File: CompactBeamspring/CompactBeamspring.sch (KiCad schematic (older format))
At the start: 32 parts, among them J1 BEAMSPRING CONNECTOR, J2 PadsToShort, J3 EXPANSION HEADER, U1 MCP4921-E, U2 LM339A, U3 74AHC595, U4 74AHC595, U5 ProMicro, U7 74AHC595

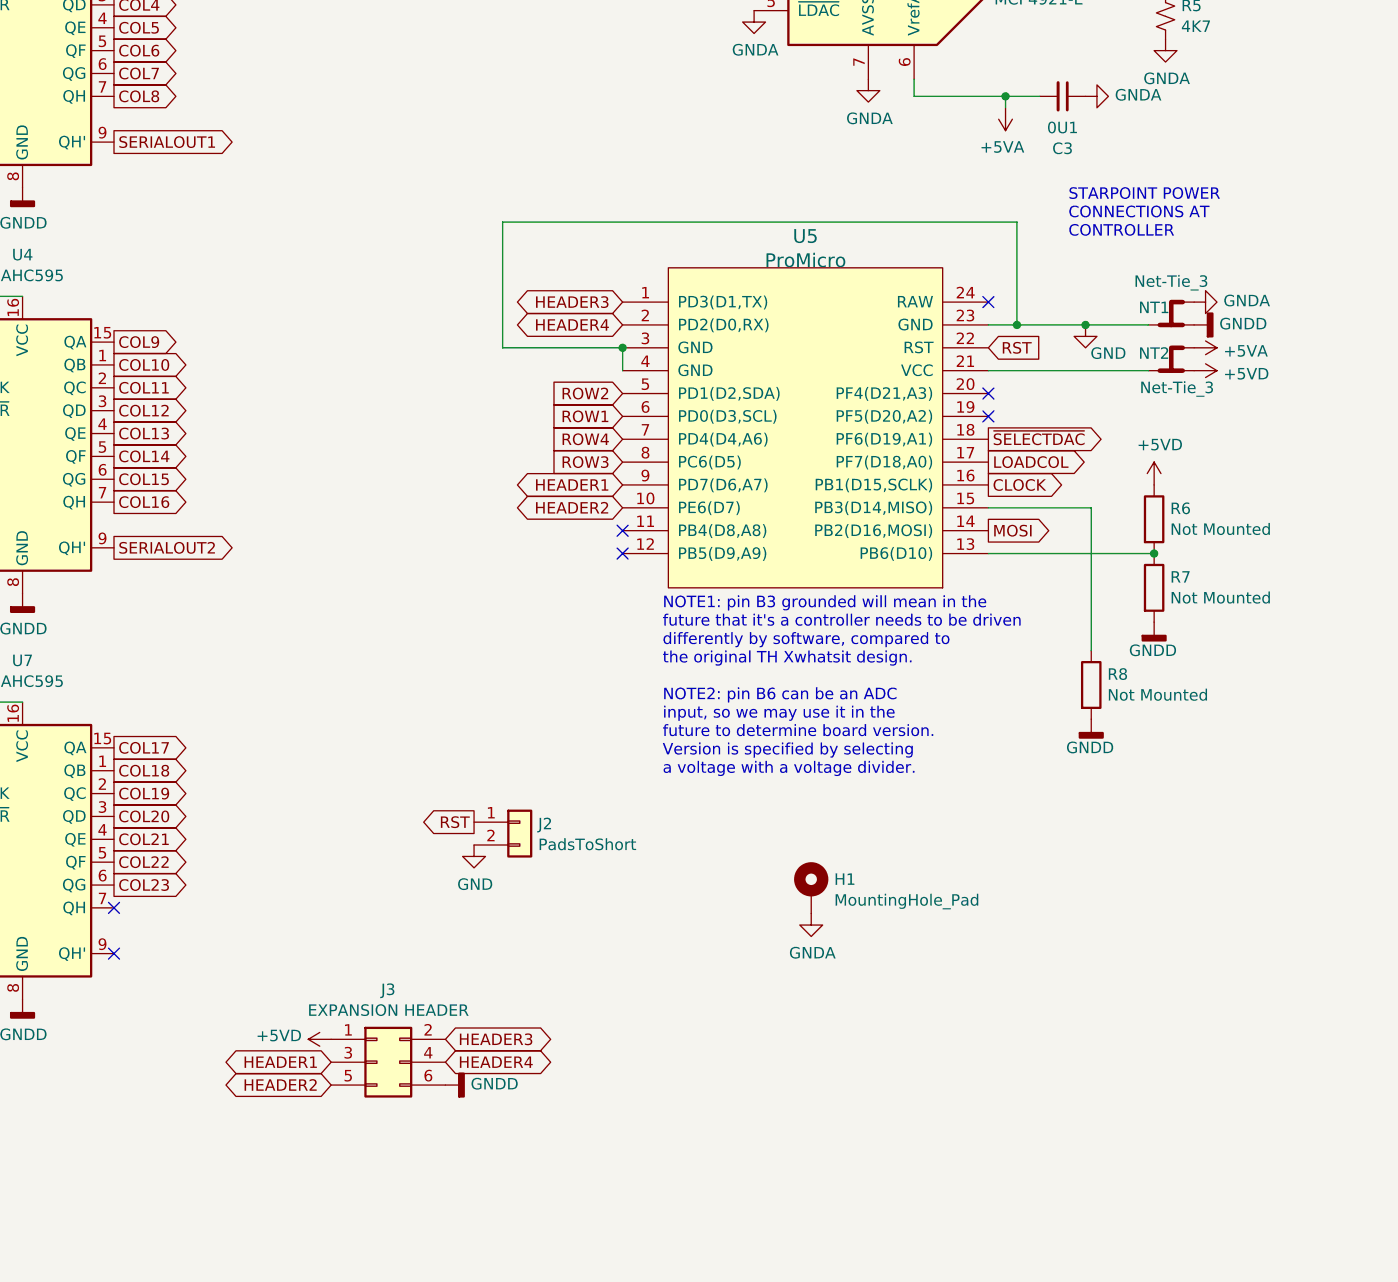
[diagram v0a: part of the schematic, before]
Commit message: Updated to rev. 1.4
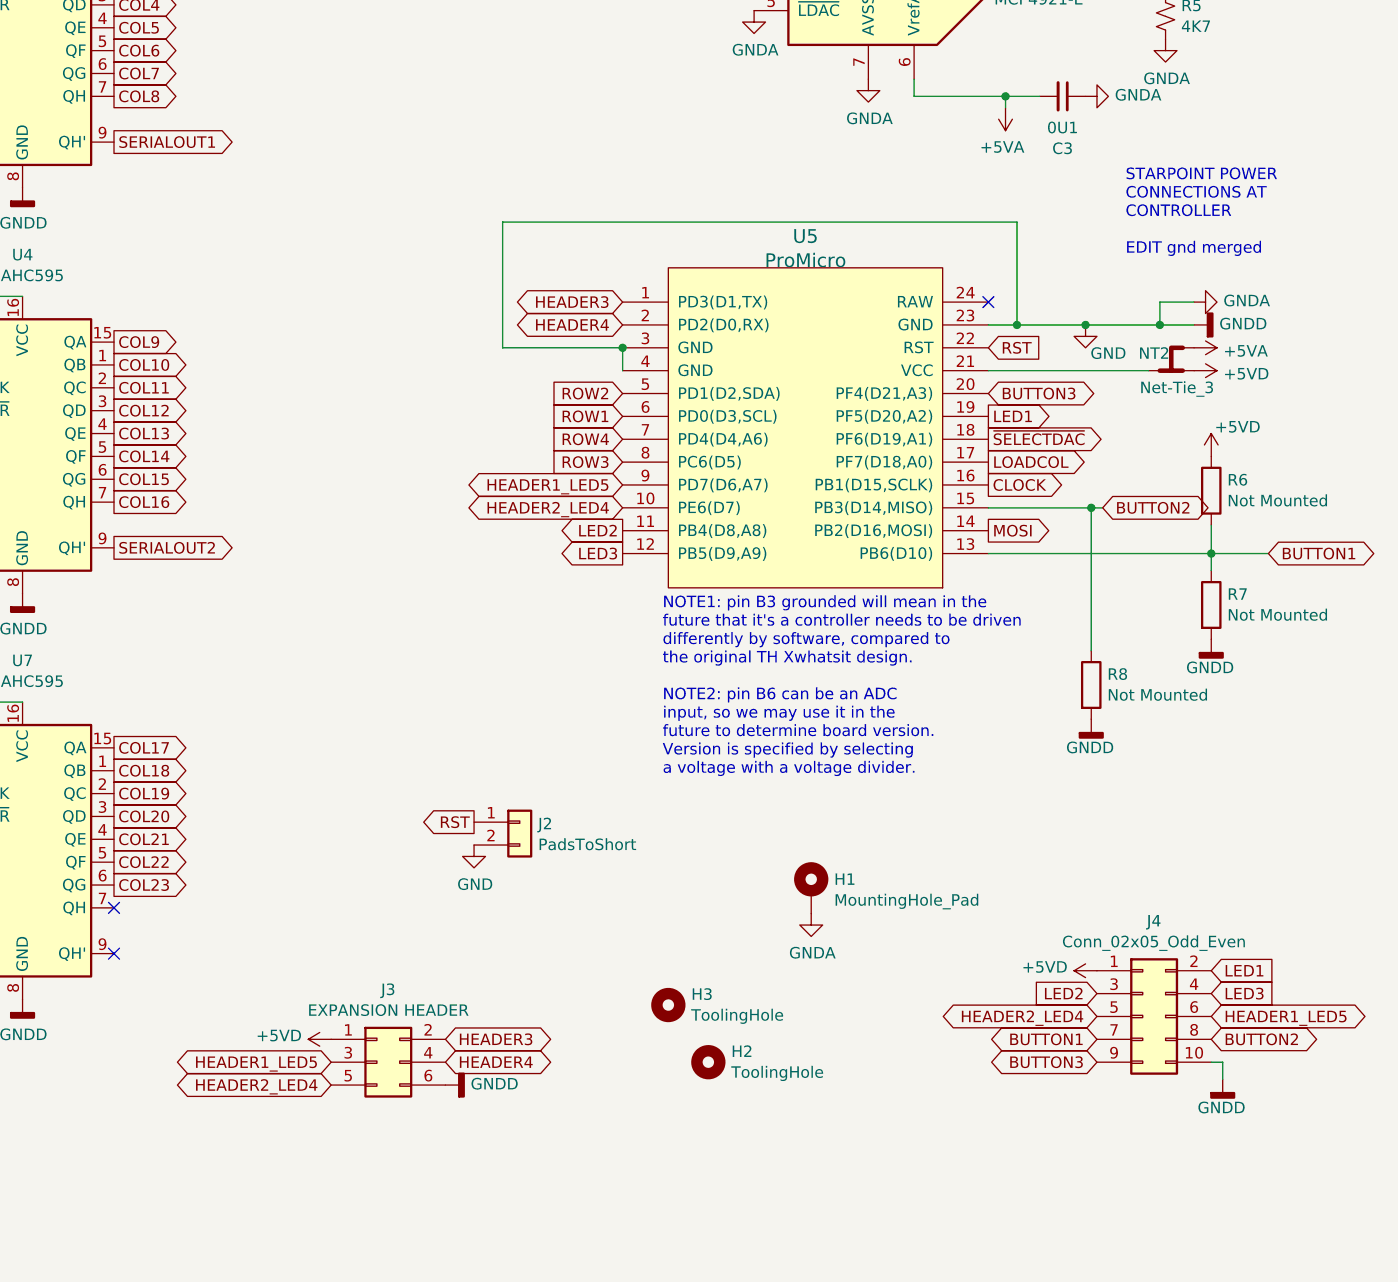
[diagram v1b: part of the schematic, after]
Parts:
- removed NT1: Net-Tie_3, NetTie:NetTie-3_THT_Pad0.3mm, symbol Device:Net-Tie_3
- added H2, H3: ToolingHole, TH-XWhatsIt:tooling_hole, symbol Mechanical:MountingHole
- added J4: Conn_02x05_Odd_Even, Connector_PinHeader_2.54mm:PinHeader_2x05_P2.54mm_Vertical, symbol Connector_Generic:Conn_02x05_Odd_Even
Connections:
- net GNDA is gone; now on net GND: C1.1, C3.1, C6.1, H1.1, R2.1, R5.1, U1.5 (~LDAC~), U1.7 (AVSS), U2.12 (V-)
- net GNDD is gone; now on net GND: C2.1, C4.1, C5.1, J1.30 (Pin_30), J1.5 (Pin_5), J3.6 (Pin_6), R7.2, R8.2, U3.13 (~OE), U3.8 (GND), U4.13 (~OE), U4.8 (GND), U7.13 (~OE), U7.8 (GND)
- net +5VD: now also J4.1 (Pin_1)
- net GND: now also J4.10 (Pin_10)
- net LED2: now reaches U5.11 (PB4(D8,A8))
- net LED2: now also J4.3 (Pin_3)
- net LED3: now reaches U5.12 (PB5(D9,A9))
- net LED3: now also J4.4 (Pin_4)
- net BUTTON1: now reaches R6.2, R7.1, U5.13 (PB6(D10))
- net BUTTON1: now also J4.7 (Pin_7)
- net BUTTON2: now reaches R8.1, U5.15 (PB3(D14,MISO))
- net BUTTON2: now also J4.8 (Pin_8)
- net LED1: now reaches U5.19 (PF5(D20,A2))
- net LED1: now also J4.2 (Pin_2)
- net BUTTON3: now reaches U5.20 (PF4(D21,A3))
- net BUTTON3: now also J4.9 (Pin_9)
- net HEADER1 renamed HEADER1_LED5
- net HEADER1_LED5: now also J4.6 (Pin_6)
- net HEADER2 renamed HEADER2_LED4
- net HEADER2_LED4: now also J4.5 (Pin_5)
- no-connect marks 8 -> 4
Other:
- note added: "STARPOINT POWER\nCONNECTIONS AT\nCONTROLLER\n\nEDIT gnd merged"
- note removed: "STARPOINT POWER\nCONNECTIONS AT\nCONTROLLER"
- moved on the sheet: R7
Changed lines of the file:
@@
 Title "Compact Beamspring Controller Based on TH Xwhatsit"
 Date "2020-01-31"
-Rev "1.3"
+Rev "1.4"
 Comp "Rainy Day Plans"
 Comment1 ""
@@
 HEADER4
 Text GLabel 7900 3575 0    50   BiDi ~ 0
-HEADER1
+HEADER1_LED5
 Text GLabel 7900 3675 0    50   BiDi ~ 0
-HEADER2
+HEADER2_LED4
 Text GLabel 7900 2775 0    50   BiDi ~ 0
 HEADER3
@@
 HEADER4
 Text GLabel 6625 6200 0    50   BiDi ~ 0
-HEADER2
+HEADER2_LED4
 Text GLabel 6625 6100 0    50   BiDi ~ 0
-HEADER1
+HEADER1_LED5
 Text Notes 3950 7750 0    50   ~ 0
 Copyright Rainy Day Plans.\nThis documentation describes Open Hardware and is licensed under the\nCERN OHL v. 1.2.\nYou may redistribute and modify this documentation under the terms of the\nCERN OHL v.1.2. (http://ohwr.org/cernohl). This documentation is distributed\nWITHOUT ANY EXPRESS OR IMPLIED WARRANTY, INCLUDING OF\nMERCHANTABILITY, SATISFACTORY QUALITY AND FITNESS FOR A\nPARTICULAR PURPOSE. Please see the CERN OHL v.1.2 for applicable\nconditions
@@
 L power:GNDD #PWR0107
 U 1 1 5F3A2D72
-P 10225 4175
-F 0 "#PWR0107" H 10225 3925 50  0001 C CNN
-F 1 "GNDD" H 10325 4050 50  0000 R CNN
-F 2 "" H 10225 4175 50  0001 C CNN
-F 3 "" H 10225 4175 50  0001 C CNN
-	1    10225 4175
+P 10475 4250
+F 0 "#PWR0107" H 10475 4000 50  0001 C CNN
+F 1 "GNDD" H 10575 4125 50  0000 R CNN
+F 2 "" H 10475 4250 50  0001 C CNN
+F 3 "" H 10475 4250 50  0001 C CNN
+	1    10475 4250
 	1    0    0    -1
 $EndComp
@@
 	2250 4275 2250 4300
 $Comp
-L Device:Net-Tie_3 NT1
-U 1 1 5F6D07D8
-P 10300 2875
-F 0 "NT1" H 10375 2800 50  0000 C CNN
-F 1 "Net-Tie_3" H 10300 2685 50  0000 C CNN
-F 2 "NetTie:NetTie-3_THT_Pad0.3mm" H 10300 2875 50  0001 C CNN
-F 3 "~" H 10300 2875 50  0001 C CNN
-	1    10300 2875
-	-1   0    0    1
-$EndComp
-$Comp
 L Device:Net-Tie_3 NT2
 U 1 1 5F6D1B28
@@
 	9625 2875 9500 2875
 $Comp
-L Device:R R6
-U 1 1 5F3A43C9
-P 10225 3725
-F 0 "R6" H 10295 3771 50  0000 L CNN
-F 1 "Not Mounted" H 10295 3680 50  0000 L CNN
-F 2 "Resistor_SMD:R_0805_2012Metric_Pad1.15x1.40mm_HandSolder" V 10155 3725 50  0001 C CNN
-F 3 "~" H 10225 3725 50  0001 C CNN
-	1    10225 3725
-	1    0    0    -1
-$EndComp
-$Comp
 L Device:R R7
 U 1 1 5F3A4C74
-P 10225 4025
-F 0 "R7" H 10295 4071 50  0000 L CNN
-F 1 "Not Mounted" H 10295 3980 50  0000 L CNN
-F 2 "Resistor_SMD:R_0805_2012Metric_Pad1.15x1.40mm_HandSolder" V 10155 4025 50  0001 C CNN
-F 3 "~" H 10225 4025 50  0001 C CNN
-	1    10225 4025
-	1    0    0    -1
-$EndComp
-Connection ~ 10225 3875
-$Comp
-L power:+5VD #PWR04
-U 1 1 5F3A9745
-P 10225 3575
-F 0 "#PWR04" H 10225 3425 50  0001 C CNN
-F 1 "+5VD" H 10150 3750 50  0000 L CNN
-F 2 "" H 10225 3575 50  0001 C CNN
-F 3 "" H 10225 3575 50  0001 C CNN
-	1    10225 3575
+P 10475 4100
+F 0 "R7" H 10545 4146 50  0000 L CNN
+F 1 "Not Mounted" H 10545 4055 50  0000 L CNN
+F 2 "Resistor_SMD:R_0805_2012Metric_Pad1.15x1.40mm_HandSolder" V 10405 4100 50  0001 C CNN
+F 3 "~" H 10475 4100 50  0001 C CNN
+	1    10475 4100
 	1    0    0    -1
 $EndComp
@@
 Wire Wire Line
 	9950 4300 9950 3675
-NoConn ~ 9500 3175
-NoConn ~ 9500 3275
-NoConn ~ 7900 3775
-NoConn ~ 7900 3875
 $Comp
 L Connector_Generic:Conn_01x02 J2
@@
 Text GLabel 7250 5050 0    50   Output ~ 0
 RST
-Wire Wire Line
-	10200 2875 9925 2875
 Connection ~ 9925 2875
 $Comp
@@
 	1    0    0    -1
 $EndComp
-Text Notes 9850 2500 0    50   ~ 0
-STARPOINT POWER\nCONNECTIONS AT\nCONTROLLER
+Text Notes 10100 2575 0    50   ~ 0
+STARPOINT POWER\nCONNECTIONS AT\nCONTROLLER\n\nEDIT gnd merged
 $Comp
 L power:GND #PWR08
@@
 	9500 3075 10200 3075
 Wire Wire Line
-	9500 3875 10225 3875
-Wire Wire Line
 	9500 3675 9950 3675
 Wire Wire Line
@@
 Wire Wire Line
 	7375 2425 9625 2425
+$Comp
+L Connector_Generic:Conn_02x05_Odd_Even J4
+U 1 1 6107AC92
+P 10175 5900
+F 0 "J4" H 10225 6317 50  0000 C CNN
+F 1 "Conn_02x05_Odd_Even" H 10225 6226 50  0000 C CNN
+F 2 "Connector_PinHeader_2.54mm:PinHeader_2x05_P2.54mm_Vertical" H 10175 5900 50  0001 C CNN
+F 3 "~" H 10175 5900 50  0001 C CNN
+	1    10175 5900
+	1    0    0    -1
+$EndComp
+Wire Wire Line
+	9925 2875 10250 2875
+Wire Wire Line
+	10250 2875 10250 2775
+Wire Wire Line
+	10250 2775 10400 2775
+Connection ~ 10250 2875
+Wire Wire Line
+	10250 2875 10400 2875
+$Comp
+L power:+5VD #PWR04
+U 1 1 61088086
+P 9975 5700
+F 0 "#PWR04" H 9975 5550 50  0001 C CNN
+F 1 "+5VD" V 9990 5828 50  0000 L CNN
+F 2 "" H 9975 5700 50  0001 C CNN
+F 3 "" H 9975 5700 50  0001 C CNN
+	1    9975 5700
+	0    -1   -1   0
+$EndComp
+Text GLabel 9500 3275 2    50   Output ~ 0
+LED1
+Text GLabel 10475 5700 2    50   Input ~ 0
+LED1
+Text GLabel 7900 3775 0    50   Output ~ 0
+LED2
+Text GLabel 7900 3875 0    50   Output ~ 0
+LED3
+Text GLabel 9975 5800 0    50   Input ~ 0
+LED2
+Text GLabel 10475 5800 2    50   Input ~ 0
+LED3
+Text GLabel 9975 5900 0    50   BiDi ~ 0
+HEADER2_LED4
+Text GLabel 10475 5900 2    50   BiDi ~ 0
+HEADER1_LED5
+Text GLabel 10725 3875 2    50   BiDi ~ 0
+BUTTON1
+Text GLabel 9975 6000 0    50   BiDi ~ 0
+BUTTON1
+Text GLabel 10000 3675 2    50   BiDi ~ 0
+BUTTON2
+Text GLabel 10475 6000 2    50   BiDi ~ 0
+BUTTON2
+Text GLabel 9500 3175 2    50   BiDi ~ 0
+BUTTON3
+Text GLabel 9975 6100 0    50   BiDi ~ 0
+BUTTON3
+$Comp
+L Device:R R6
+U 1 1 610C2CCF
+P 10475 3600
+F 0 "R6" H 10545 3646 50  0000 L CNN
+F 1 "Not Mounted" H 10545 3555 50  0000 L CNN
+F 2 "Resistor_SMD:R_0805_2012Metric_Pad1.15x1.40mm_HandSolder" V 10405 3600 50  0001 C CNN
+F 3 "~" H 10475 3600 50  0001 C CNN
+	1    10475 3600
+	1    0    0    -1
+$EndComp
+$Comp
+L power:GNDD #PWR0103
+U 1 1 610D5B38
+P 10525 6175
+F 0 "#PWR0103" H 10525 5925 50  0001 C CNN
+F 1 "GNDD" H 10625 6050 50  0000 R CNN
+F 2 "" H 10525 6175 50  0001 C CNN
+F 3 "" H 10525 6175 50  0001 C CNN
+	1    10525 6175
+	1    0    0    -1
+$EndComp
+Wire Wire Line
+	10475 6100 10525 6100
+Wire Wire Line
+	10525 6100 10525 6175
+Wire Wire Line
+	10000 3675 9950 3675
+Connection ~ 9950 3675
+Wire Wire Line
+	9500 3875 10475 3875
+Wire Wire Line
+	10475 3750 10475 3875
+Connection ~ 10475 3875
+Wire Wire Line
+	10475 3875 10725 3875
+Wire Wire Line
+	10475 3875 10475 3950
+$Comp
+L power:+5VD #PWR0110
+U 1 1 6112E48C
+P 10475 3450
+F 0 "#PWR0110" H 10475 3300 50  0001 C CNN
+F 1 "+5VD" H 10490 3578 50  0000 L CNN
+F 2 "" H 10475 3450 50  0001 C CNN
+F 3 "" H 10475 3450 50  0001 C CNN
+	1    10475 3450
+	1    0    0    -1
+$EndComp
+$Comp
+L Mechanical:MountingHole H2
+U 1 1 611D25F7
+P 8275 6100
+F 0 "H2" H 8375 6146 50  0000 L CNN
+F 1 "ToolingHole" H 8375 6055 50  0000 L CNN
+F 2 "TH-XWhatsIt:tooling_hole" H 8275 6100 50  0001 C CNN
+F 3 "~" H 8275 6100 50  0001 C CNN
+	1    8275 6100
+	1    0    0    -1
+$EndComp
+$Comp
+L Mechanical:MountingHole H3
+U 1 1 611DB711
+P 8100 5850
+F 0 "H3" H 8200 5896 50  0000 L CNN
+F 1 "ToolingHole" H 8200 5805 50  0000 L CNN
+F 2 "TH-XWhatsIt:tooling_hole" H 8100 5850 50  0001 C CNN
+F 3 "~" H 8100 5850 50  0001 C CNN
+	1    8100 5850
+	1    0    0    -1
+$EndComp
 $EndSCHEMATC

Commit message: Updated shift register and 100k resistor LCSC part numbers
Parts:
- R10, R11, R12, R9: LCSC C17407 -> C149504
- U3, U4, U7: LCSC C5520 -> C2682116
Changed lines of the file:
@@
 F 2 "Package_SO:SOIC-16_3.9x9.9mm_P1.27mm" H 5275 1575 50  0001 C CNN
 F 3 "https://assets.nexperia.com/documents/data-sheet/74HC_HCT595.pdf" H 5275 1575 50  0001 C CNN
-F 4 "C5520" H 5275 1575 50  0001 C CNN "LCSC"
+F 4 "C2682116" H 5275 1575 50  0001 C CNN "LCSC"
 	1    5275 1575
 	1    0    0    -1
@@
 F 2 "Package_SO:SOIC-16_3.9x9.9mm_P1.27mm" H 5275 3350 50  0001 C CNN
 F 3 "https://assets.nexperia.com/documents/data-sheet/74HC_HCT595.pdf" H 5275 3350 50  0001 C CNN
-F 4 "C5520" H 5275 3350 50  0001 C CNN "LCSC"
+F 4 "C2682116" H 5275 3350 50  0001 C CNN "LCSC"
 	1    5275 3350
 	1    0    0    -1
@@
 F 2 "Package_SO:SOIC-16_3.9x9.9mm_P1.27mm" H 5275 5125 50  0001 C CNN
 F 3 "https://assets.nexperia.com/documents/data-sheet/74HC_HCT595.pdf" H 5275 5125 50  0001 C CNN
-F 4 "C5520" H 5275 5125 50  0001 C CNN "LCSC"
+F 4 "C2682116" H 5275 5125 50  0001 C CNN "LCSC"
 	1    5275 5125
 	1    0    0    -1
@@
 F 2 "Resistor_SMD:R_0805_2012Metric_Pad1.15x1.40mm_HandSolder" V 1380 1325 50  0001 C CNN
 F 3 "~" H 1450 1325 50  0001 C CNN
-F 4 "C17407" H 1450 1325 50  0001 C CNN "LCSC"
+F 4 "C149504" H 1450 1325 50  0001 C CNN "LCSC"
 	1    1450 1325
 	1    0    0    -1
@@
 F 2 "Resistor_SMD:R_0805_2012Metric_Pad1.15x1.40mm_HandSolder" V 1380 1925 50  0001 C CNN
 F 3 "~" H 1450 1925 50  0001 C CNN
-F 4 "C17407" H 1450 1925 50  0001 C CNN "LCSC"
+F 4 "C149504" H 1450 1925 50  0001 C CNN "LCSC"
 	1    1450 1925
 	1    0    0    -1
@@
 F 2 "Resistor_SMD:R_0805_2012Metric_Pad1.15x1.40mm_HandSolder" V 1380 2525 50  0001 C CNN
 F 3 "~" H 1450 2525 50  0001 C CNN
-F 4 "C17407" H 1450 2525 50  0001 C CNN "LCSC"
+F 4 "C149504" H 1450 2525 50  0001 C CNN "LCSC"
 	1    1450 2525
 	1    0    0    -1
@@
 F 2 "Resistor_SMD:R_0805_2012Metric_Pad1.15x1.40mm_HandSolder" V 1380 3125 50  0001 C CNN
 F 3 "~" H 1450 3125 50  0001 C CNN
-F 4 "C17407" H 1450 3125 50  0001 C CNN "LCSC"
+F 4 "C149504" H 1450 3125 50  0001 C CNN "LCSC"
 	1    1450 3125
 	1    0    0    -1

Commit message: Revert part of commit 'Updated 100k resistor and shift register LCSC part numbers' (the shift register BOM changes only)
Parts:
- U3, U4, U7: LCSC C2682116 -> C5520
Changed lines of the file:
@@
 F 2 "Package_SO:SOIC-16_3.9x9.9mm_P1.27mm" H 5275 1575 50  0001 C CNN
 F 3 "https://assets.nexperia.com/documents/data-sheet/74HC_HCT595.pdf" H 5275 1575 50  0001 C CNN
-F 4 "C2682116" H 5275 1575 50  0001 C CNN "LCSC"
+F 4 "C5520" H 5275 1575 50  0001 C CNN "LCSC"
 	1    5275 1575
 	1    0    0    -1
@@
 F 2 "Package_SO:SOIC-16_3.9x9.9mm_P1.27mm" H 5275 3350 50  0001 C CNN
 F 3 "https://assets.nexperia.com/documents/data-sheet/74HC_HCT595.pdf" H 5275 3350 50  0001 C CNN
-F 4 "C2682116" H 5275 3350 50  0001 C CNN "LCSC"
+F 4 "C5520" H 5275 3350 50  0001 C CNN "LCSC"
 	1    5275 3350
 	1    0    0    -1
@@
 F 2 "Package_SO:SOIC-16_3.9x9.9mm_P1.27mm" H 5275 5125 50  0001 C CNN
 F 3 "https://assets.nexperia.com/documents/data-sheet/74HC_HCT595.pdf" H 5275 5125 50  0001 C CNN
-F 4 "C2682116" H 5275 5125 50  0001 C CNN "LCSC"
+F 4 "C5520" H 5275 5125 50  0001 C CNN "LCSC"
 	1    5275 5125
 	1    0    0    -1
